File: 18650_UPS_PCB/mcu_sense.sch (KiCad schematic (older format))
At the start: 20 parts, among them SW2 5_Way_Tactile, SW3 PWR MODE, U7 SSD1306_128_32, U8 INA219AxD, U9 STM32F030F4Px

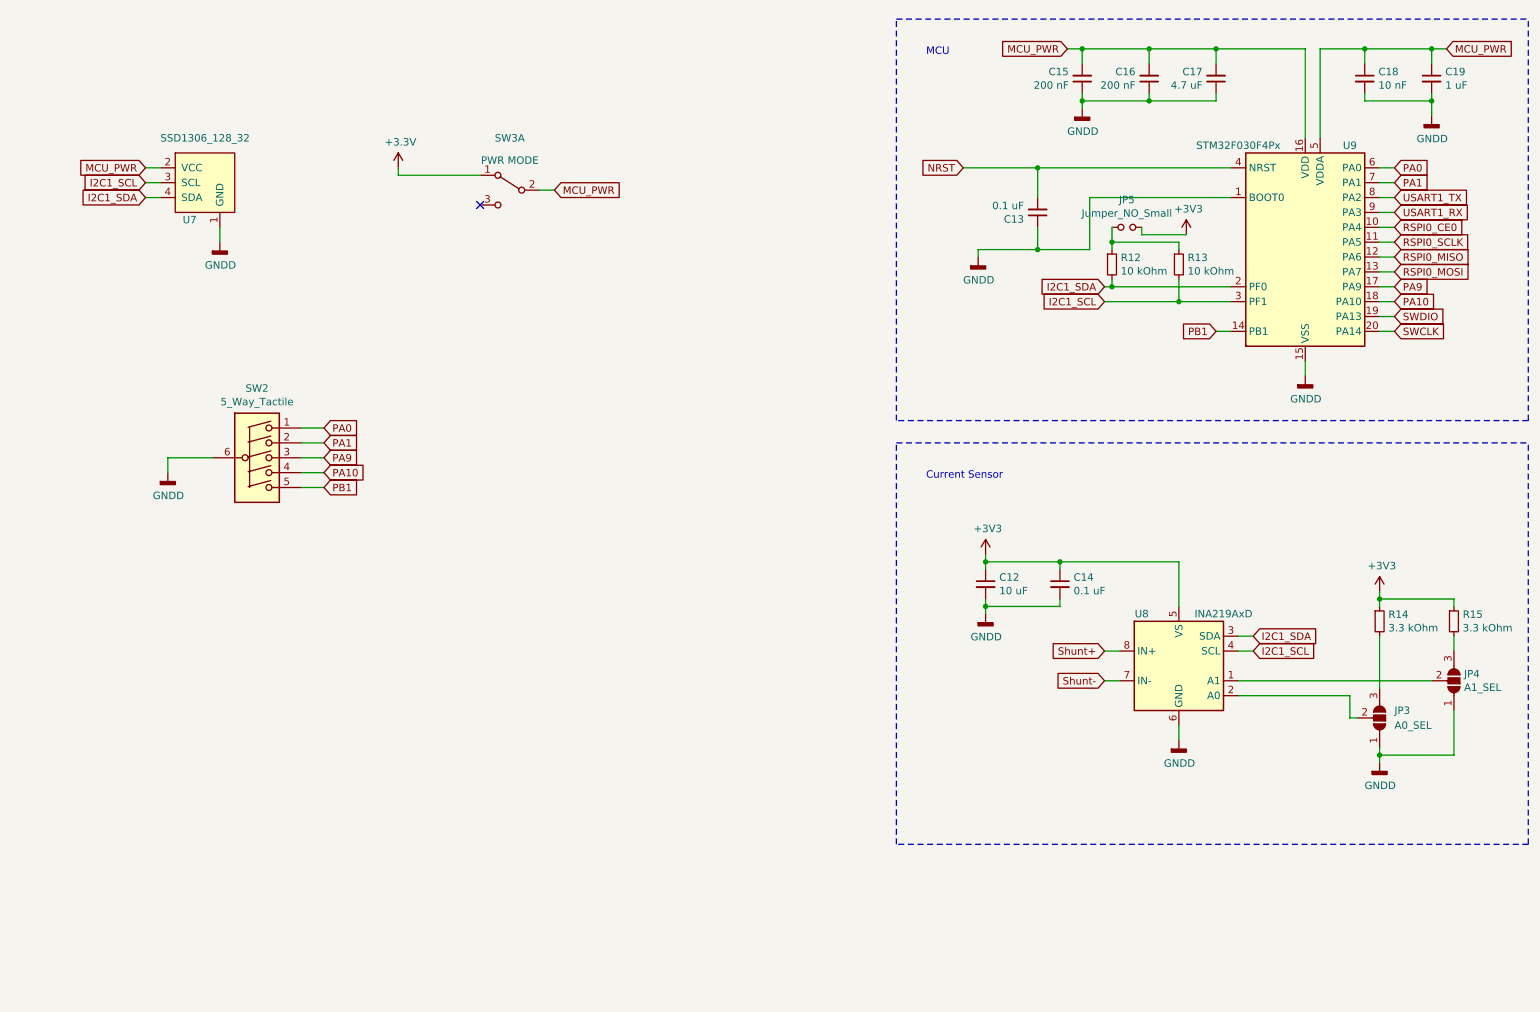
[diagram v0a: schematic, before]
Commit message: first routing done
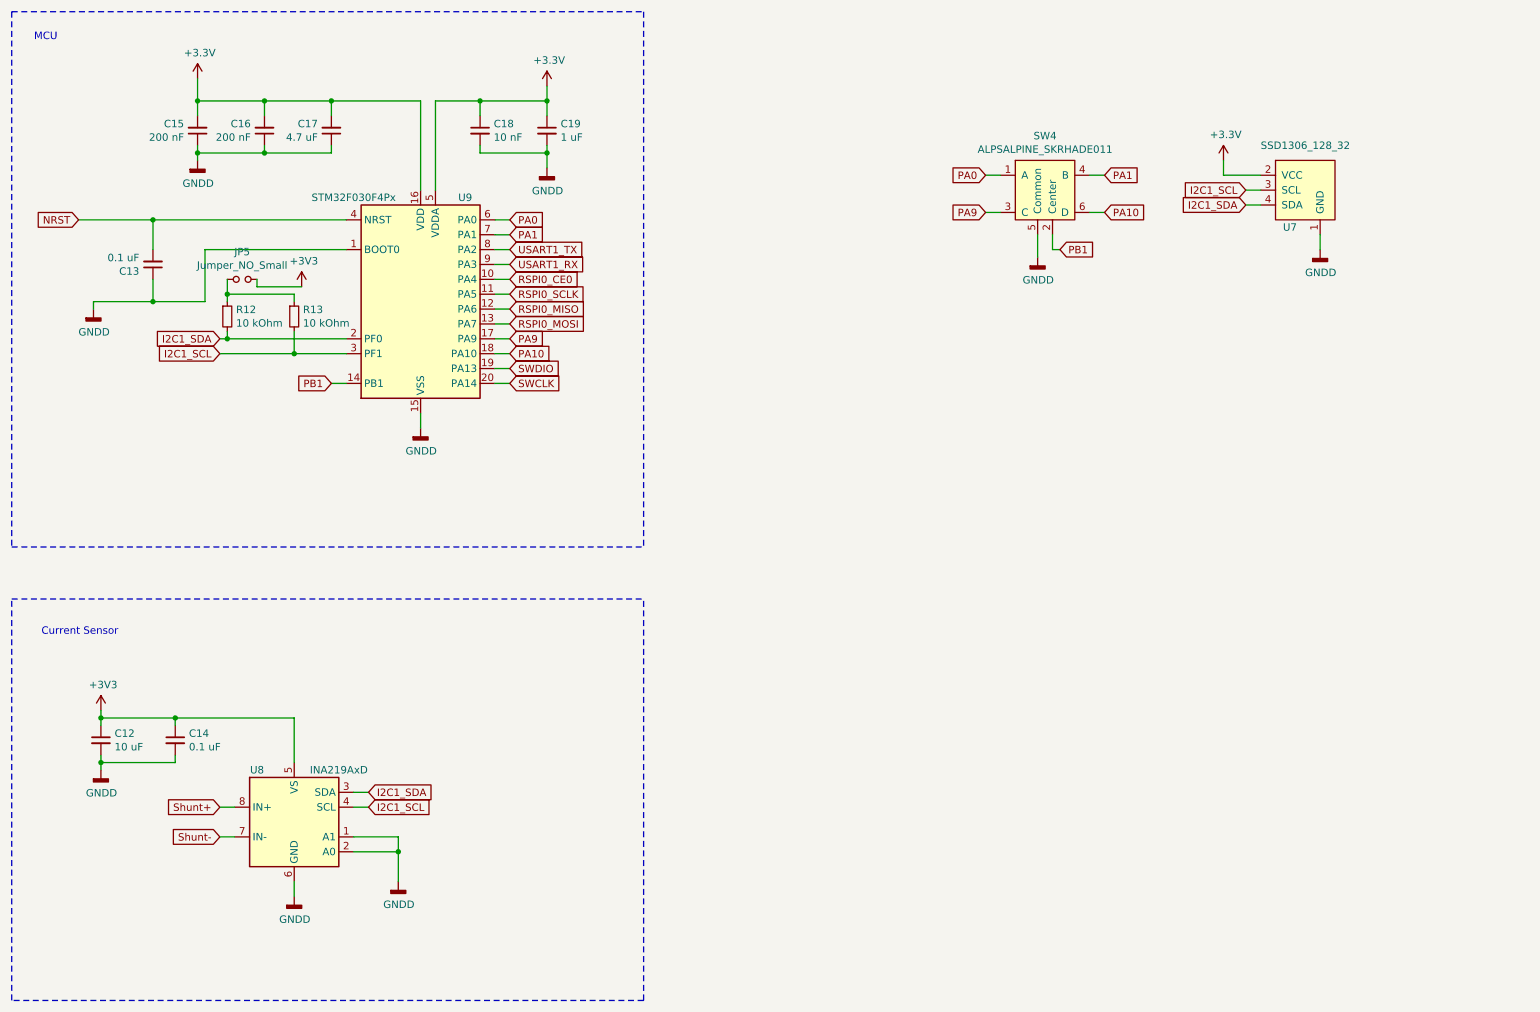
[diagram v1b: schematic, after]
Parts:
- removed JP3: A0_SEL, Jumper:SolderJumper-3_P1.3mm_Open_RoundedPad1.0x1.5mm, symbol Jumper:SolderJumper_3_Open
- removed JP4: A1_SEL, Jumper:SolderJumper-3_P1.3mm_Open_RoundedPad1.0x1.5mm, symbol Jumper:SolderJumper_3_Open
- removed R14, R15: 3.3 kOhm, Resistor_SMD:R_0603_1608Metric, symbol Device:R_Small
- removed SW2: 5_Way_Tactile, CUSTOM_FOOTPRINTS:5_Way_Tactical, symbol CUSTOM_PARTS:5_Way_Tactile
- removed SW3: PWR MODE, Button_Switch_THT:SW_CuK_OS102011MA1QN1_SPDT_Angled, symbol Switch:SW_DPDT_x2
- added SW4: ALPSALPINE_SKRHADE011, CUSTOM_FOOTPRINTS:SKRHADE011, symbol CUSTOM_PARTS:ALPSALPINE_SKRHADE011
- U7: footprint Connector_PinSocket_2.54mm:PinSocket_1x04_P2.54mm_Vertical -> Connector_PinHeader_2.54mm:PinHeader_1x04_P2.54mm_Vertical_SMD_Pin1Left
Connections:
- net MCU_PWR is gone; now on net +3V3: C15.2, C16.2, C17.2, C18.1, C19.1, U7.2 (VCC), U9.16 (VDD), U9.5 (VDDA)
- net GNDD: now also U8.1 (A1), U8.2 (A0), SW4.5 (Common)
- net PA0: now also SW4.1 (A)
- net PA1: now also SW4.4 (B)
- net PA10: now also SW4.6 (D)
- net PA9: now also SW4.3 (C)
- net PB1: now also SW4.2 (Center)
- no-connect marks 1 -> 0
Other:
- moved on the sheet: C12, C13, C14, C15, C16, C17, C18, C19, JP5, R12, R13, U7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
